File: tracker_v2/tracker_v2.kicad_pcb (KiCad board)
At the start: 2 copper layers, 72.9 x 21.6 mm, 26 parts, among them J1 USB_C_Receptacle_PowerOnly_6P, Q1 DMG9926UDM-7, U1 XIAO-ESP32-C6-SMD, U2 LIS3DH, U3 DW01A, U4 INA226AIDGSR, U5 TP4056-42-ESOP8

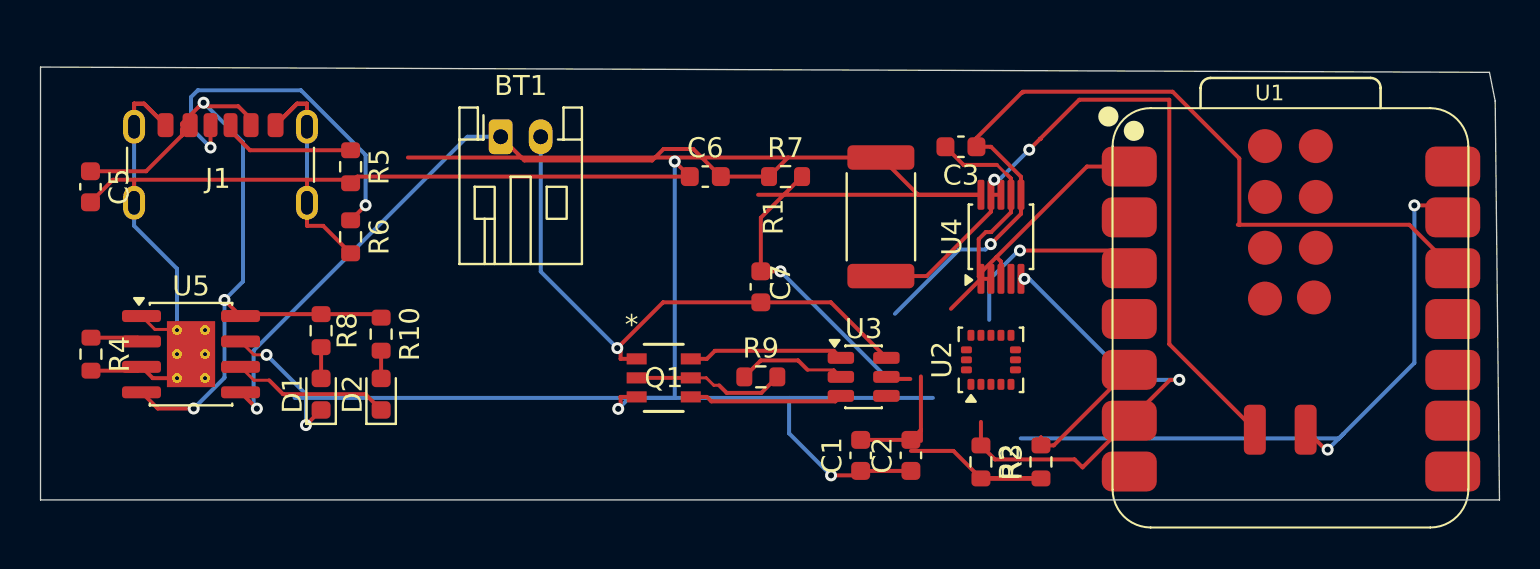
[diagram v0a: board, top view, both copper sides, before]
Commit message: completed v2 routing
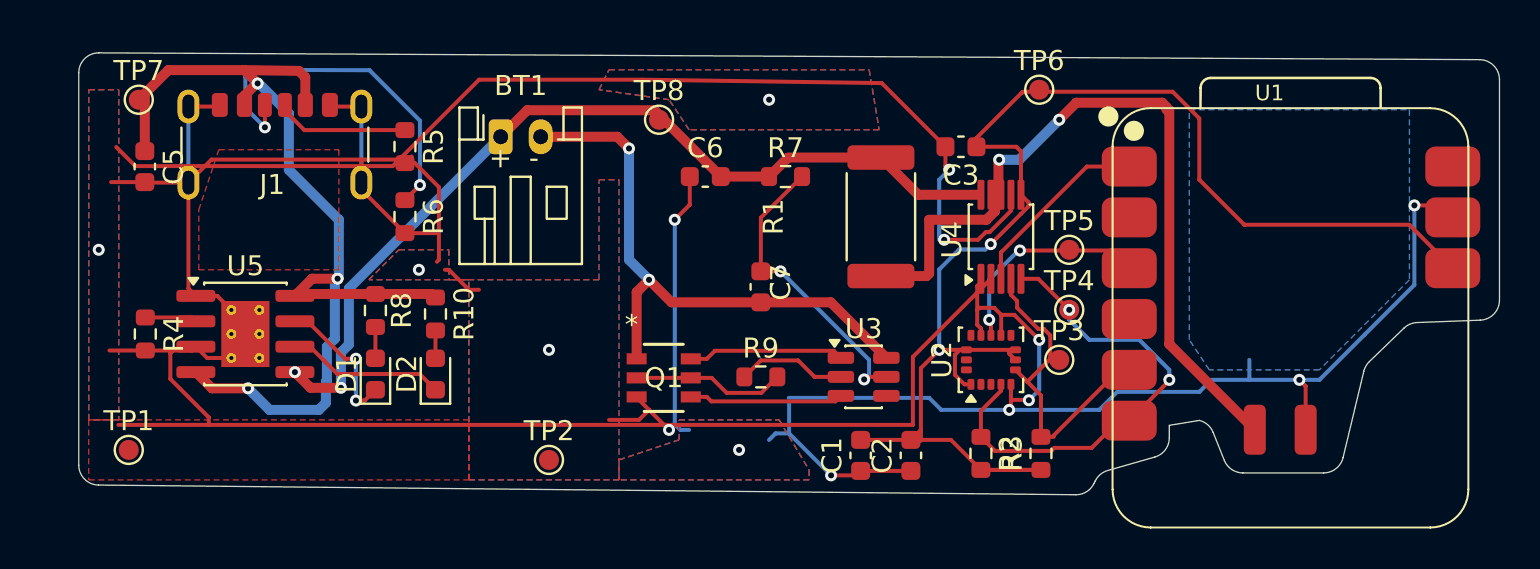
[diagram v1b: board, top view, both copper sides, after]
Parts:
- added TP1: TestPoint, TestPoint:TestPoint_Pad_D1.0mm, F.Cu at (124.5, 92.0)
- added TP2: TestPoint, TestPoint:TestPoint_Pad_D1.0mm, F.Cu at (145.5, 92.5)
- added TP3: TestPoint, TestPoint:TestPoint_Pad_D1.0mm, F.Cu at (171.0, 87.5)
- added TP4: TestPoint, TestPoint:TestPoint_Pad_D1.0mm, F.Cu at (171.5, 85.0)
- added TP5: TestPoint, TestPoint:TestPoint_Pad_D1.0mm, F.Cu at (171.5, 82.0)
- added TP6: TestPoint, TestPoint:TestPoint_Pad_D1.0mm, F.Cu at (170.0, 74.0)
- added TP7: TestPoint, TestPoint:TestPoint_Pad_D1.0mm, F.Cu at (125.0, 74.5)
- added TP8: TestPoint, TestPoint:TestPoint_Pad_D1.0mm, F.Cu at (151.0, 75.5)
- moved J1 2.90 mm to (131.8, 77.8)
- moved R5 2.90 mm to (138.3, 76.8)
- moved R6 2.90 mm to (138.3, 80.3)
- moved R4 2.90 mm to (125.3, 86.2)
- moved C5 2.90 mm to (125.3, 77.8)
- moved U5 2.90 mm to (130.3, 86.2)
- moved D1 2.90 mm to (136.8, 88.2)
- moved D2 2.90 mm to (139.8, 88.2)
- moved R10 2.90 mm to (139.8, 85.2)
- moved R8 2.90 mm to (136.8, 85.0)
- moved R2 0.43 mm to (167.1, 92.2)
- moved R3 0.43 mm to (170.1, 92.2)
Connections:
- U2 pad 7: unconnected-(U2-SDO-Pad7) -> 3v3
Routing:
- net GND: track 182.4 -> 246.9 mm, vias 5 -> 12
- net /Charging_and_Battery/BAT+: track 77.5 -> 45.9 mm, vias 1 -> 2
- net USB_VBUS: track 39.2 -> 51.0 mm
- net 3v3: track 60.4 -> 70.7 mm, vias 1 -> 2
- net SDA: track 6.78 -> 16.2 mm
- net (no net): track 0.00 -> 2.11 mm, vias 0 -> 3
- net Net-(U1-D0): track 10.9 -> 9.51 mm
- net Net-(U3-VCC): track 16.5 -> 15.2 mm, vias 1 -> 2
- net SCL: track 23.2 -> 24.3 mm
- net /Shunt_Output: track 37.7 -> 38.7 mm
- net Net-(U1-D2): track 10.0 -> 10.8 mm, vias 1 -> 2
- net /Charging_and_Battery/BAT-: track 29.1 -> 29.3 mm, vias 1 -> 2
- added copper zone on B.Cu, net GND
- added copper zone on F.Cu, net GND
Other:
- board size 72.9 x 21.6 mm -> 71 x 22.1 mm
- board text added: "+"
- board text added: "-"
